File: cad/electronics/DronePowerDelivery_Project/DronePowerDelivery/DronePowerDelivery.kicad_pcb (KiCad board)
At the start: 4 copper layers, 52.6 x 56.4 mm, 42 parts, among them J1 Conn_01x05_Socket, J2 Conn_01x02_Socket, J3 Conn_01x04_Pin, J4 Conn_01x02_Socket, Q1 Q_NMOS_GDS, Q2 Q_NMOS_GDS, Q3 Q_PMOS_GSD, SW1 SW_Push, U1 BQ76920PW

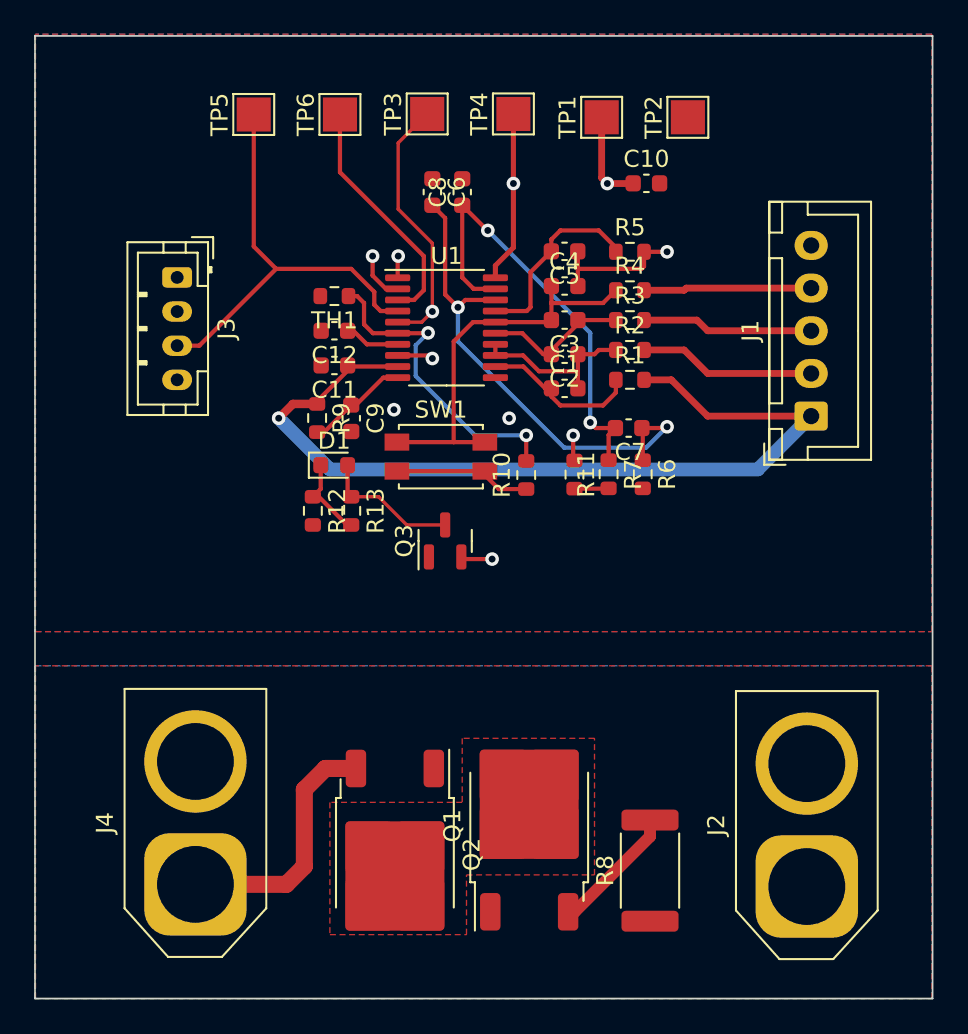
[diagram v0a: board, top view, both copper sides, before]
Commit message: Finalied Rev1 Layout
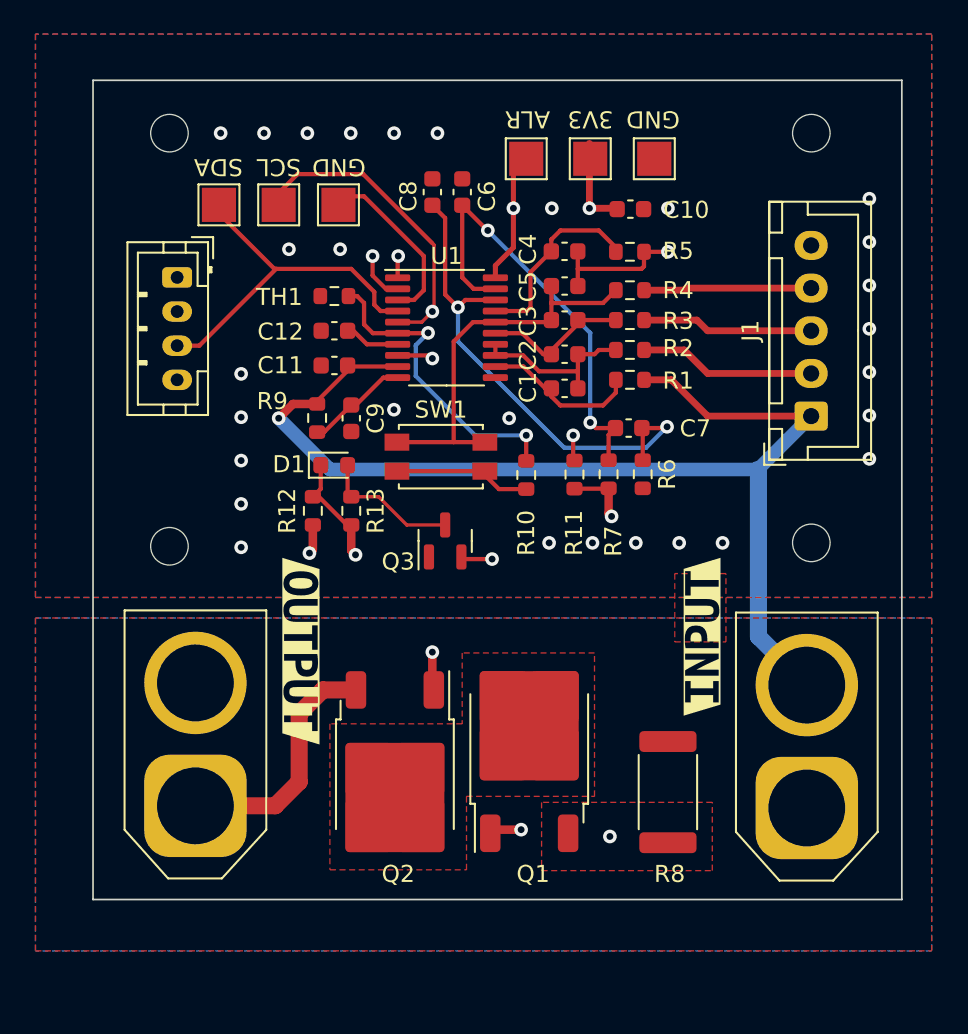
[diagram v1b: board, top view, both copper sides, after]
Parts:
- added G***: LOGO, LOGO, B.Cu at (105.5, 95.8)
- added REF**: MountingHole_2.2mm_M2_ISO14580, MountingHole:MountingHole_2.2mm_M2_ISO14580, F.Cu at (85.6, 100.0)
- added REF**: MountingHole_2.2mm_M2_ISO14580, MountingHole:MountingHole_2.2mm_M2_ISO14580, F.Cu at (123.2, 99.8)
- added REF**: MountingHole_2.2mm_M2_ISO14580, MountingHole:MountingHole_2.2mm_M2_ISO14580, F.Cu at (123.2, 75.8)
- added REF**: MountingHole_2.2mm_M2_ISO14580, MountingHole:MountingHole_2.2mm_M2_ISO14580, F.Cu at (85.6, 75.8)
- added kibuzzard-64ABA4C5: G***, kibuzzard-64ABA4C5, F.Cu at (116.8, 105.3)
- added kibuzzard-64ABA514: G***, kibuzzard-64ABA514, F.Cu at (93.3, 106.1)
- moved TP3 10.2 mm to (92.0, 80.0)
- moved TP5 5.67 mm to (88.5, 80.0)
- moved TP6 5.29 mm to (95.5, 80.0)
- moved R8 4.72 mm to (114.8, 114.4), turned to -90 degrees
- moved J2 4.60 mm to (122.9, 115.3)
- moved J4 4.60 mm to (87.1, 115.2)
- moved Q2 4.60 mm to (98.8, 113.5)
- moved Q1 4.60 mm to (106.7, 111.8)
- moved TP2 3.13 mm to (114.0, 77.3)
- moved TP4 2.73 mm to (106.5, 77.3)
- moved TP1 2.52 mm to (110.2, 77.3)
- moved C10 1.78 mm to (112.6, 80.2)
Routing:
- net /CellMonitor/DSG: track 20.9 -> 47.2 mm, vias 2 -> 3
- net /PACK_L: track 14.9 -> 36.6 mm, vias 0 -> 1
- net /PACK_H: track 52.9 -> 66.8 mm
- net /CellMonitor/Q1_SRC: track 9.59 -> 22.5 mm, vias 0 -> 2
- net /CellMonitor/IN_PROT: track 4.98 -> 16.6 mm, vias 0 -> 2
- net /SDA: track 25.8 -> 21.4 mm
- net GNDREF: track 22.3 -> 18.6 mm, vias 3 -> 30
- net /SCL: track 34.7 -> 37.5 mm
- net /REGOUT: track 22.1 -> 20.4 mm
- net /ALERT: track 40.2 -> 38.5 mm
- added copper zone on F.Cu, net /CellMonitor/Q1_SRC
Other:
- board size 52.6 x 56.4 mm -> 47.4 x 48 mm
- board text added: "3V3"
- board text added: "ALR"
- board text added: "BatPD Rev. 1 M. Singh Jul. 2023"
- board text added: "GND"
- board text added: "SCL"
- board text added: "SDA"
